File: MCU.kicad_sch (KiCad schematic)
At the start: 15 parts, among them U3 STM32F405RGT6, Y1 12MHz

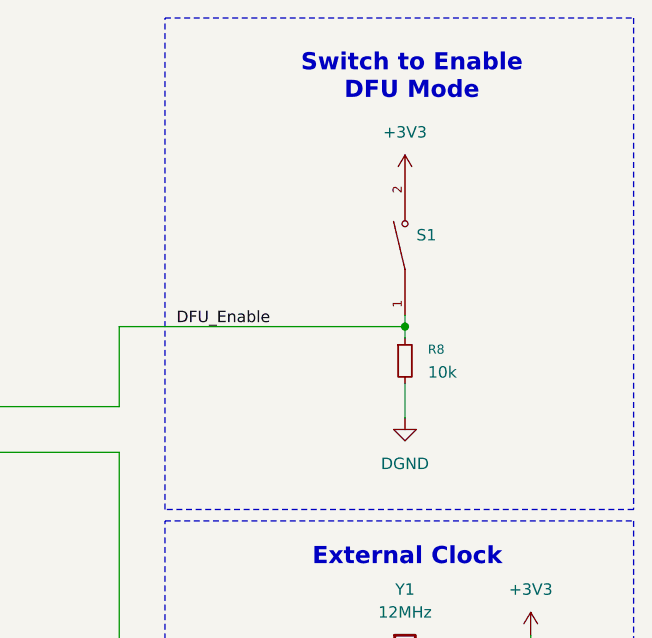
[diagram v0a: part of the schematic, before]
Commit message: Layout Draft Complete
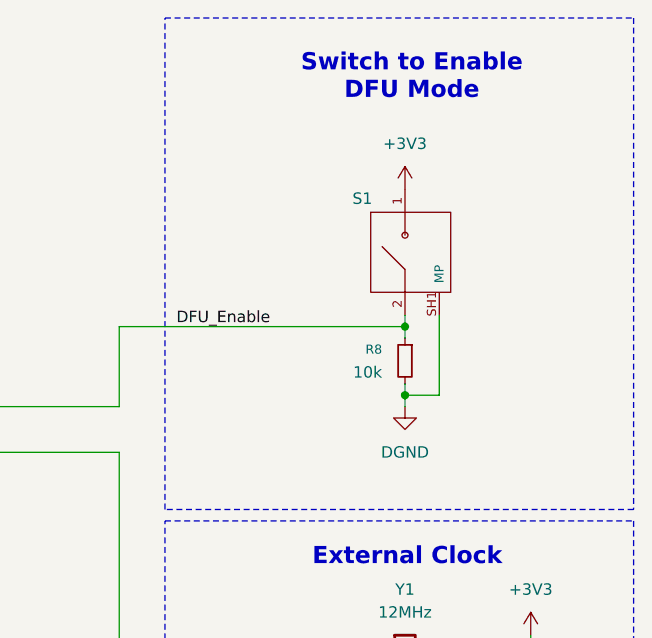
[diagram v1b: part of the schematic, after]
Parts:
- S1: value TS32-7-35-BK-B-260-RA-SMT-TR -> NO; MPN (none) -> TS32-7-35-BK-B-260-RA-SMT-TR; Manufacturer (none) -> Same Sky
- Y1: footprint Crystal:Crystal_SMD_Abracon_ABM8AIG-4Pin_3.2x2.5mm -> KSE_passive:Crystal_SMD_Abracon_ABM8AIG-4Pin_3.2x2.5mm
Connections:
- net +3V3: now also S1.1; no longer S1.2
- net DFU_Enable: now also S1.2; no longer S1.1
- net DGND: now also S1.SH1 (MP), S1.SH2 (MP)
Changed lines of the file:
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@@
 	)
 	(junction
+		(at 257.81 55.88)
+		(diameter 0)
+		(color 0 0 0 0)
+	)
+	(junction
 		(at 257.81 48.26)
 		(diameter 0)
@@
 	(wire
 		(pts
+			(xy 257.81 55.88) (xy 257.81 57.15)
+		)
+		(stroke
+			(width 0)
+			(type default)
+		)
+	)
+	(wire
+		(pts
 			(xy 257.81 90.17) (xy 257.81 95.25)
 		)
@@
 	(wire
 		(pts
+			(xy 261.62 46.99) (xy 261.62 55.88)
+		)
+		(stroke
+			(width 0)
+			(type default)
+		)
+	)
+	(wire
+		(pts
 			(xy 143.51 29.21) (xy 143.51 44.45)
 		)
@@
 	(wire
 		(pts
-			(xy 257.81 54.61) (xy 257.81 58.42)
+			(xy 257.81 54.61) (xy 257.81 55.88)
 		)
 		(stroke
@@
 		)
 	)
+	(wire
+		(pts
+			(xy 261.62 55.88) (xy 257.81 55.88)
+		)
+		(stroke
+			(width 0)
+			(type default)
+		)
+	)
 	(label "DFU_Enable"
 		(at 232.41 48.26 0)
@@
 	(symbol
 		(lib_id "KSE_sensors:TS32-7-35-BK-B-260-RA-SMT-TR")
-		(at 257.81 39.37 90)
+		(at 257.81 39.37 0)
 		(unit 1)
 		(exclude_from_sim no)
@@
 		(on_board yes)
 		(dnp no)
-		(fields_autoplaced yes)
 		(property "Reference" "S1"
-			(at 259.08 38.0999 90)
+			(at 251.968 34.036 0)
 			(effects
 				(font
 					(size 1.27 1.27)
 				)
-				(justify right)
+				(justify left)
 			)
 		)
-		(property "Value" "TS32-7-35-BK-B-260-RA-SMT-TR"
-			(at 259.08 40.6399 90)
+		(property "Value" "NO"
+			(at 253.492 33.782 0)
 			(effects
 				(font
@@
 			)
 		)
-		(property "Datasheet" ""
+		(property "Datasheet" "https://eu.mouser.com/datasheet/3/6118/1/ts32.pdf"
 			(at 257.81 39.37 0)
 			(effects
@@
 			)
 		)
-		(property "Description" ""
+		(property "Description" "Tactile Switch SPST-NO Side Actuated Surface Mount, Right Angle"
 			(at 257.81 39.37 0)
 			(effects
@@
 			)
 		)
+		(property "Manufacturer" "Same Sky"
+			(at 259.08 71.628 0)
+			(effects
+				(font
+					(size 1.27 1.27)
+				)
+				(justify bottom)
+				(hide yes)
+			)
+		)
+		(property "MPN" "TS32-7-35-BK-B-260-RA-SMT-TR"
+			(at 258.826 65.532 0)
+			(effects
+				(font
+					(size 1.27 1.27)
+				)
+				(justify bottom)
+				(hide yes)
+			)
+		)
 		(pin "2"
 		)
 		(pin "1"
 		)
+		(pin "SH1"
+		)
+		(pin "SH2"
+		)
 		(instances
 			(project "FCU3"
@@
 	(symbol
 		(lib_id "power:+3.3V")
-		(at 257.81 31.75 0)
+		(at 257.81 33.02 0)
 		(mirror y)
 		(unit 1)
@@
 		(fields_autoplaced yes)
 		(property "Reference" "#PWR014"
-			(at 257.81 35.56 0)
+			(at 257.81 36.83 0)
 			(effects
 				(font
@@
 		)
 		(property "Value" "+3V3"
-			(at 257.81 26.67 0)
+			(at 257.81 27.94 0)
 			(effects
 				(font
@@
 		)
 		(property "Footprint" ""
-			(at 257.81 31.75 0)
+			(at 257.81 33.02 0)
 			(effects
 				(font
@@
 		)
 		(property "Datasheet" ""
-			(at 257.81 31.75 0)
+			(at 257.81 33.02 0)
 			(effects
 				(font
@@
 		)
 		(property "Description" "Power symbol creates a global label with name \"+3.3V\""
-			(at 257.81 31.75 0)
+			(at 257.81 33.02 0)
 			(effects
 				(font
@@
 			)
 		)
-		(property "Footprint" "Crystal:Crystal_SMD_Abracon_ABM8AIG-4Pin_3.2x2.5mm"
+		(property "Footprint" "KSE_passive:Crystal_SMD_Abracon_ABM8AIG-4Pin_3.2x2.5mm"
 			(at 257.81 85.09 0)
 			(effects
@@
 		(lib_id "KSE_Resistors:R_Small")
 		(at 257.81 52.07 0)
+		(mirror y)
 		(unit 1)
 		(exclude_from_sim no)
@@
 		(on_board yes)
 		(dnp no)
-		(fields_autoplaced yes)
 		(property "Reference" "R8"
-			(at 260.35 50.7999 0)
+			(at 255.27 50.7999 0)
 			(effects
 				(font
@@
 		)
 		(property "Value" "10k"
-			(at 260.35 53.3399 0)
+			(at 255.27 53.3399 0)
 			(effects
 				(font
@@
 	(symbol
 		(lib_id "power:GND2")
-		(at 257.81 58.42 0)
+		(at 257.81 57.15 0)
 		(mirror y)
 		(unit 1)
@@
 		(fields_autoplaced yes)
 		(property "Reference" "#PWR016"
-			(at 257.81 64.77 0)
+			(at 257.81 63.5 0)
 			(effects
 				(font
@@
 		)
 		(property "Value" "DGND"
-			(at 257.81 63.5 0)
+			(at 257.81 62.23 0)
 			(effects
 				(font
@@
 		)
 		(property "Footprint" ""
-			(at 257.81 58.42 0)
+			(at 257.81 57.15 0)
 			(effects
 				(font
@@
 		)
 		(property "Datasheet" ""
-			(at 257.81 58.42 0)
+			(at 257.81 57.15 0)
 			(effects
 				(font
@@
 		)
 		(property "Description" "Power symbol creates a global label with name \"GND2\" , ground"
-			(at 257.81 58.42 0)
+			(at 257.81 57.15 0)
 			(effects
 				(font

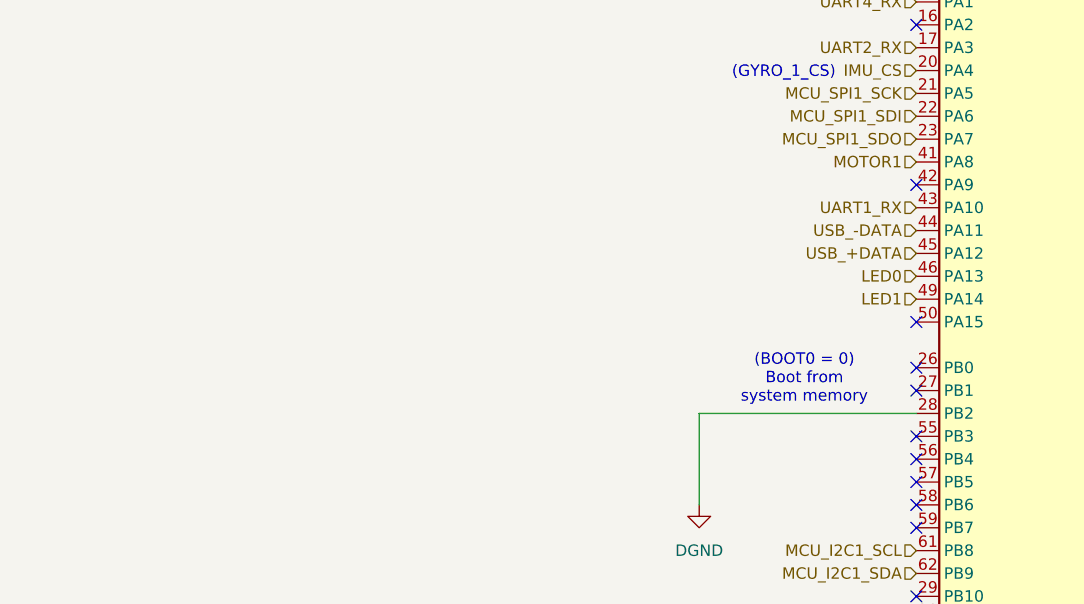
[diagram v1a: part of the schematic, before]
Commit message: DRC/ERC Remaining
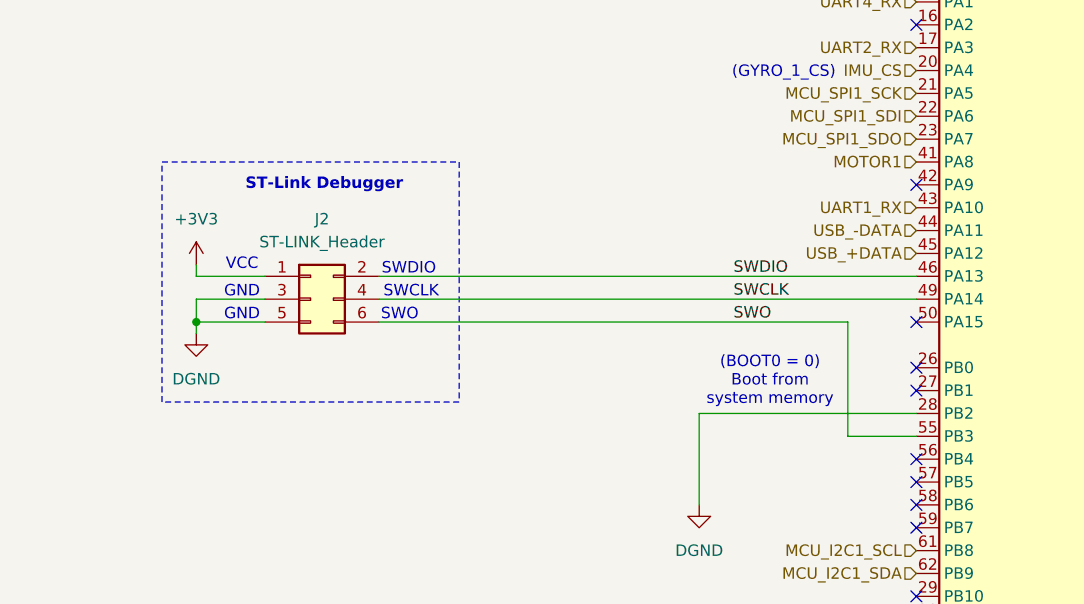
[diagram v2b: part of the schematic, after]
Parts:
- added J2: ST-LINK_Header, Connector_PinHeader_1.27mm:PinHeader_2x03_P1.27mm_Vertical_SMD, symbol KSE_connectors:ST-LINK_Header
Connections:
- net +3V3: now also J2.1 (Pin_1)
- net DGND: now also J2.3 (Pin_3), J2.5 (Pin_5)
- net SWO: now reaches U3.55 (PB3)
- net SWO: now also J2.6 (Pin_6)
- net LED0 renamed SWDIO
- net SWDIO: now also J2.2 (Pin_2)
- net LED1 renamed SWCLK
- net SWCLK: now also J2.4 (Pin_4)
- no-connect marks 28 -> 27
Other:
- note added: "GND"
- note added: "ST-Link Debugger"
- note added: "SWCLK"
- note added: "SWDIO"
- note added: "SWO"
- note added: "VCC"
